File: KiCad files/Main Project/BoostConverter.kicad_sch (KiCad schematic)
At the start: 9 parts, among them Q1 Si2319CDS, U1 2108

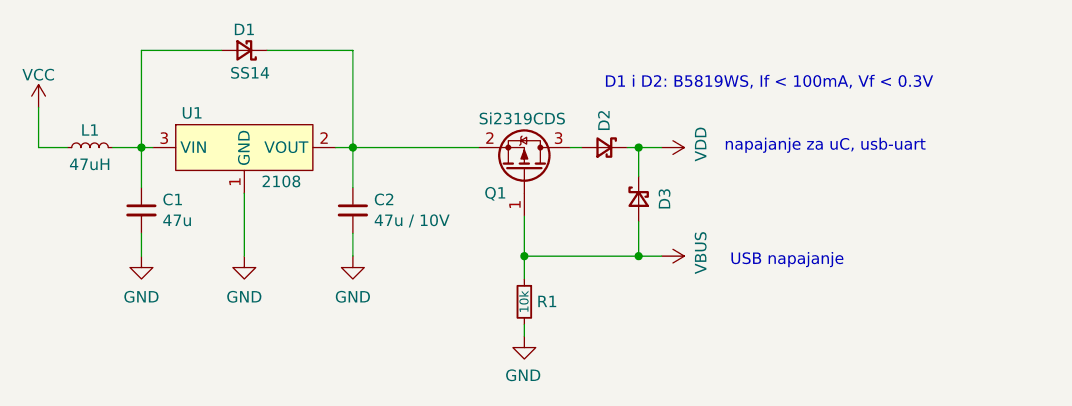
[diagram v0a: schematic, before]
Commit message: update
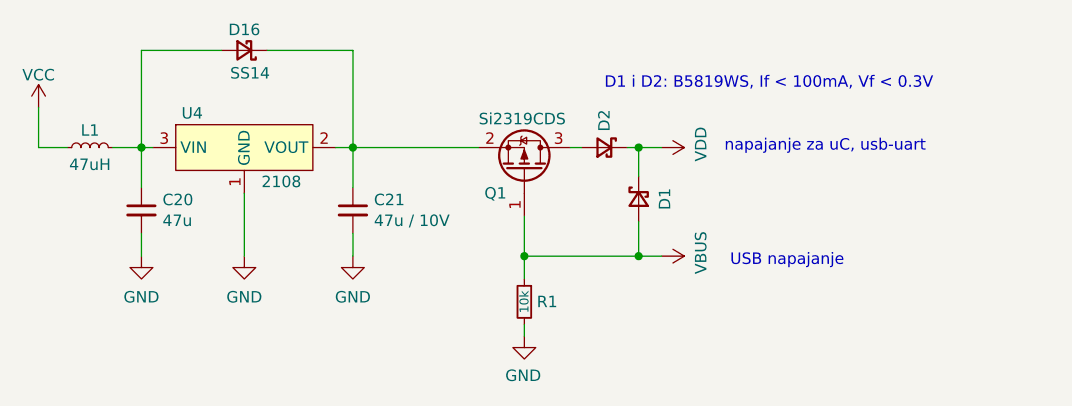
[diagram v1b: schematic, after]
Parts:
- renumbered C1 to C20, C2 to C21, D3 to D1, D1 to D16, U1 to U4
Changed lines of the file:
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@@
   (symbol (lib_id "power:VBUS") (at 139.065 93.345 270) (mirror x) (unit 1)
     (in_bom yes) (on_board yes)
-    (property "Reference" "#PWR09" (id 0) (at 135.255 93.345 0)
+    (property "Reference" "#PWR01" (id 0) (at 135.255 93.345 0)
       (effects (font (size 1.27 1.27)) hide)
     )
@@
   (symbol (lib_id "Device:D_Schottky_Small") (at 136.525 86.995 90) (mirror x) (unit 1)
     (in_bom yes) (on_board yes)
-    (property "Reference" "D3" (id 0) (at 139.446 86.995 0))
+    (property "Reference" "D1" (id 0) (at 139.446 86.995 0))
     (property "Value" "B5819WS" (id 1) (at 139.4714 86.995 0)
       (effects (font (size 1.27 1.27)) hide)
@@
   (symbol (lib_id "power:GND") (at 123.825 102.235 0) (mirror y) (unit 1)
     (in_bom yes) (on_board yes)
-    (property "Reference" "#PWR010" (id 0) (at 123.825 108.585 0)
+    (property "Reference" "#PWR02" (id 0) (at 123.825 108.585 0)
       (effects (font (size 1.27 1.27)) hide)
     )
@@
   (symbol (lib_id "power:VDD") (at 139.065 81.28 270) (mirror x) (unit 1)
     (in_bom yes) (on_board yes)
-    (property "Reference" "#PWR05" (id 0) (at 135.255 81.28 0)
+    (property "Reference" "#PWR03" (id 0) (at 135.255 81.28 0)
       (effects (font (size 1.27 1.27)) hide)
     )
@@
   (symbol (lib_id "power:GND") (at 81.28 93.345 0) (unit 1)
     (in_bom yes) (on_board yes) (fields_autoplaced)
-    (property "Reference" "#PWR06" (id 0) (at 81.28 99.695 0)
+    (property "Reference" "#PWR0101" (id 0) (at 81.28 99.695 0)
       (effects (font (size 1.27 1.27)) hide)
     )
@@
   (symbol (lib_id "power:VCC") (at 69.85 76.835 0) (unit 1)
     (in_bom yes) (on_board yes) (fields_autoplaced)
-    (property "Reference" "#PWR04" (id 0) (at 69.85 80.645 0)
+    (property "Reference" "#PWR0102" (id 0) (at 69.85 80.645 0)
       (effects (font (size 1.27 1.27)) hide)
     )
@@
   (symbol (lib_id "power:GND") (at 104.775 93.345 0) (unit 1)
     (in_bom yes) (on_board yes) (fields_autoplaced)
-    (property "Reference" "#PWR08" (id 0) (at 104.775 99.695 0)
+    (property "Reference" "#PWR0104" (id 0) (at 104.775 99.695 0)
       (effects (font (size 1.27 1.27)) hide)
     )
@@
   (symbol (lib_id "CNLJS-symbols:2108") (at 92.71 81.28 0) (unit 1)
     (in_bom yes) (on_board yes)
-    (property "Reference" "U1" (id 0) (at 85.725 77.47 0)
+    (property "Reference" "U4" (id 0) (at 85.725 77.47 0)
       (effects (font (size 1.27 1.27)) (justify left))
     )
@@
   (symbol (lib_id "power:GND") (at 92.71 93.345 0) (unit 1)
     (in_bom yes) (on_board yes) (fields_autoplaced)
-    (property "Reference" "#PWR07" (id 0) (at 92.71 99.695 0)
+    (property "Reference" "#PWR0103" (id 0) (at 92.71 99.695 0)
       (effects (font (size 1.27 1.27)) hide)
     )
@@
   (symbol (lib_id "Device:C_Small") (at 104.775 88.265 0) (unit 1)
     (in_bom yes) (on_board yes)
-    (property "Reference" "C2" (id 0) (at 107.1118 87.0966 0)
+    (property "Reference" "C21" (id 0) (at 107.1118 87.0966 0)
       (effects (font (size 1.27 1.27)) (justify left))
     )
@@
   (symbol (lib_id "Device:C_Small") (at 81.28 88.265 0) (unit 1)
     (in_bom yes) (on_board yes)
-    (property "Reference" "C1" (id 0) (at 83.6168 87.0966 0)
+    (property "Reference" "C20" (id 0) (at 83.6168 87.0966 0)
       (effects (font (size 1.27 1.27)) (justify left))
     )
@@
   (symbol (lib_id "Device:D_Schottky_Small") (at 92.71 70.485 180) (unit 1)
     (in_bom yes) (on_board yes)
-    (property "Reference" "D1" (id 0) (at 92.71 68.199 0))
+    (property "Reference" "D16" (id 0) (at 92.71 68.199 0))
     (property "Value" "SS14" (id 1) (at 93.345 73.025 0))
     (property "Footprint" "Diode_SMD:D_SMA" (id 2) (at 92.71 70.485 90)

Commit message: shematic update
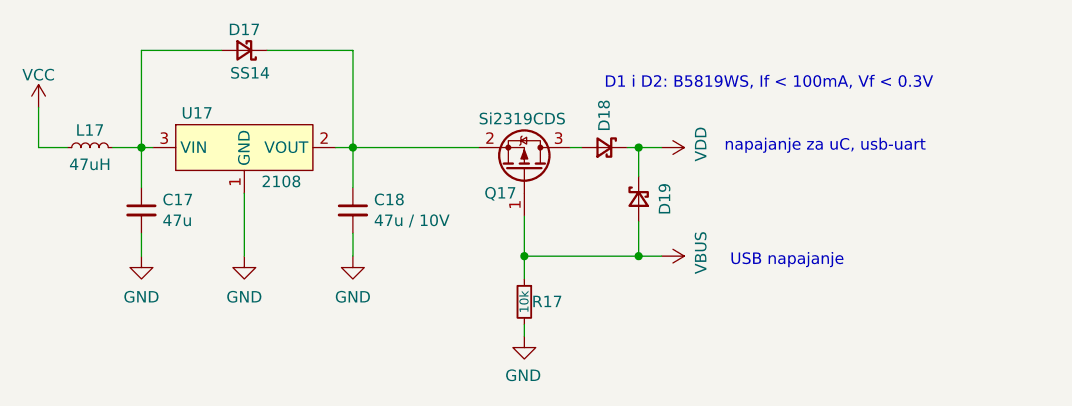
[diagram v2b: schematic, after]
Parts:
- renumbered C20 to C17, C21 to C18, D16 to D17, D2 to D18, D1 to D19, L1 to L17, Q1 to Q17, R1 to R17, U4 to U17
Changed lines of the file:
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@@
   (symbol (lib_id "power:VBUS") (at 139.065 93.345 270) (mirror x) (unit 1)
     (in_bom yes) (on_board yes)
-    (property "Reference" "#PWR01" (id 0) (at 135.255 93.345 0)
+    (property "Reference" "#PWR025" (id 0) (at 135.255 93.345 0)
       (effects (font (size 1.27 1.27)) hide)
     )
@@
   (symbol (lib_id "Device:D_Schottky_Small") (at 136.525 86.995 90) (mirror x) (unit 1)
     (in_bom yes) (on_board yes)
-    (property "Reference" "D1" (id 0) (at 139.446 86.995 0))
+    (property "Reference" "D19" (id 0) (at 139.446 86.995 0))
     (property "Value" "B5819WS" (id 1) (at 139.4714 86.995 0)
       (effects (font (size 1.27 1.27)) hide)
@@
   (symbol (lib_id "Device:R_Small") (at 123.825 98.425 0) (mirror y) (unit 1)
     (in_bom yes) (on_board yes)
-    (property "Reference" "R1" (id 0) (at 126.365 98.425 0))
+    (property "Reference" "R17" (id 0) (at 126.365 98.425 0))
     (property "Value" "10k" (id 1) (at 123.825 98.425 90)
       (effects (font (size 0.9906 0.9906)))
@@
   (symbol (lib_id "power:GND") (at 123.825 102.235 0) (mirror y) (unit 1)
     (in_bom yes) (on_board yes)
-    (property "Reference" "#PWR02" (id 0) (at 123.825 108.585 0)
+    (property "Reference" "#PWR026" (id 0) (at 123.825 108.585 0)
       (effects (font (size 1.27 1.27)) hide)
     )
@@
   (symbol (lib_id "Transistor_FET:Si2319CDS") (at 123.825 83.82 270) (mirror x) (unit 1)
     (in_bom yes) (on_board yes)
-    (property "Reference" "Q1" (id 0) (at 119.38 86.36 90)
+    (property "Reference" "Q17" (id 0) (at 119.38 86.36 90)
       (effects (font (size 1.27 1.27)) (justify left))
     )
@@
   (symbol (lib_id "Device:D_Schottky_Small") (at 132.715 81.28 0) (mirror y) (unit 1)
     (in_bom yes) (on_board yes)
-    (property "Reference" "D2" (id 0) (at 132.715 79.502 90)
+    (property "Reference" "D18" (id 0) (at 132.715 79.502 90)
       (effects (font (size 1.27 1.27)) (justify left))
     )
@@
   (symbol (lib_id "power:VDD") (at 139.065 81.28 270) (mirror x) (unit 1)
     (in_bom yes) (on_board yes)
-    (property "Reference" "#PWR03" (id 0) (at 135.255 81.28 0)
+    (property "Reference" "#PWR021" (id 0) (at 135.255 81.28 0)
       (effects (font (size 1.27 1.27)) hide)
     )
@@
   (symbol (lib_id "power:GND") (at 81.28 93.345 0) (unit 1)
     (in_bom yes) (on_board yes) (fields_autoplaced)
-    (property "Reference" "#PWR0101" (id 0) (at 81.28 99.695 0)
+    (property "Reference" "#PWR022" (id 0) (at 81.28 99.695 0)
       (effects (font (size 1.27 1.27)) hide)
     )
@@
   (symbol (lib_id "Device:L_Small") (at 75.565 81.28 90) (unit 1)
     (in_bom yes) (on_board yes)
-    (property "Reference" "L1" (id 0) (at 75.565 79.375 90))
+    (property "Reference" "L17" (id 0) (at 75.565 79.375 90))
     (property "Value" "47uH" (id 1) (at 75.565 83.185 90))
     (property "Footprint" "CNLJS:L_Taiyo-Yuden_NR-50xx" (id 2) (at 75.565 81.28 0)
@@
   (symbol (lib_id "power:VCC") (at 69.85 76.835 0) (unit 1)
     (in_bom yes) (on_board yes) (fields_autoplaced)
-    (property "Reference" "#PWR0102" (id 0) (at 69.85 80.645 0)
+    (property "Reference" "#PWR020" (id 0) (at 69.85 80.645 0)
       (effects (font (size 1.27 1.27)) hide)
     )
@@
   (symbol (lib_id "power:GND") (at 104.775 93.345 0) (unit 1)
     (in_bom yes) (on_board yes) (fields_autoplaced)
-    (property "Reference" "#PWR0104" (id 0) (at 104.775 99.695 0)
+    (property "Reference" "#PWR024" (id 0) (at 104.775 99.695 0)
       (effects (font (size 1.27 1.27)) hide)
     )
@@
   (symbol (lib_id "CNLJS-symbols:2108") (at 92.71 81.28 0) (unit 1)
     (in_bom yes) (on_board yes)
-    (property "Reference" "U4" (id 0) (at 85.725 77.47 0)
+    (property "Reference" "U17" (id 0) (at 85.725 77.47 0)
       (effects (font (size 1.27 1.27)) (justify left))
     )
@@
   (symbol (lib_id "power:GND") (at 92.71 93.345 0) (unit 1)
     (in_bom yes) (on_board yes) (fields_autoplaced)
-    (property "Reference" "#PWR0103" (id 0) (at 92.71 99.695 0)
+    (property "Reference" "#PWR023" (id 0) (at 92.71 99.695 0)
       (effects (font (size 1.27 1.27)) hide)
     )
@@
   (symbol (lib_id "Device:C_Small") (at 104.775 88.265 0) (unit 1)
     (in_bom yes) (on_board yes)
-    (property "Reference" "C21" (id 0) (at 107.1118 87.0966 0)
+    (property "Reference" "C18" (id 0) (at 107.1118 87.0966 0)
       (effects (font (size 1.27 1.27)) (justify left))
     )
@@
   (symbol (lib_id "Device:C_Small") (at 81.28 88.265 0) (unit 1)
     (in_bom yes) (on_board yes)
-    (property "Reference" "C20" (id 0) (at 83.6168 87.0966 0)
+    (property "Reference" "C17" (id 0) (at 83.6168 87.0966 0)
       (effects (font (size 1.27 1.27)) (justify left))
     )
@@
   (symbol (lib_id "Device:D_Schottky_Small") (at 92.71 70.485 180) (unit 1)
     (in_bom yes) (on_board yes)
-    (property "Reference" "D16" (id 0) (at 92.71 68.199 0))
+    (property "Reference" "D17" (id 0) (at 92.71 68.199 0))
     (property "Value" "SS14" (id 1) (at 93.345 73.025 0))
     (property "Footprint" "Diode_SMD:D_SMA" (id 2) (at 92.71 70.485 90)

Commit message: update
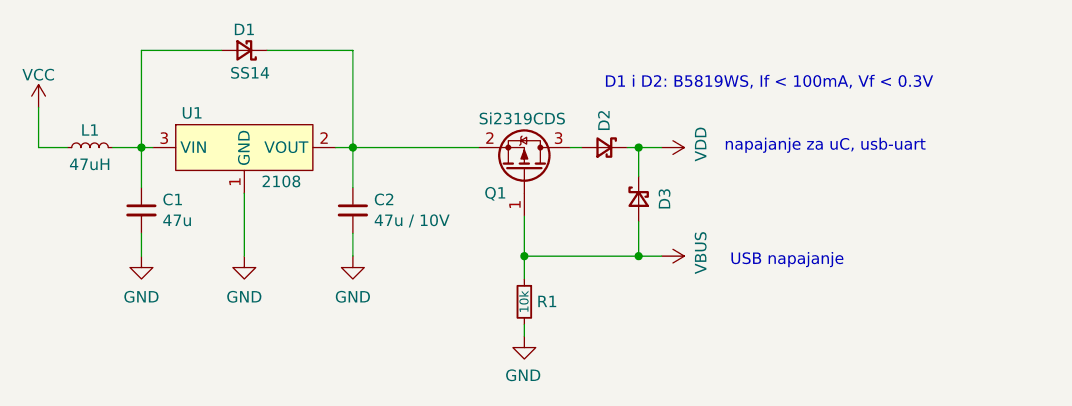
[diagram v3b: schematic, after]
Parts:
- renumbered C17 to C1, C18 to C2, D17 to D1, D18 to D2, D19 to D3, L17 to L1, Q17 to Q1, R17 to R1, U17 to U1
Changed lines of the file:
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@@
   (symbol (lib_id "power:VBUS") (at 139.065 93.345 270) (mirror x) (unit 1)
     (in_bom yes) (on_board yes)
-    (property "Reference" "#PWR025" (id 0) (at 135.255 93.345 0)
+    (property "Reference" "#PWR09" (id 0) (at 135.255 93.345 0)
       (effects (font (size 1.27 1.27)) hide)
     )
@@
   (symbol (lib_id "Device:D_Schottky_Small") (at 136.525 86.995 90) (mirror x) (unit 1)
     (in_bom yes) (on_board yes)
-    (property "Reference" "D19" (id 0) (at 139.446 86.995 0))
+    (property "Reference" "D3" (id 0) (at 139.446 86.995 0))
     (property "Value" "B5819WS" (id 1) (at 139.4714 86.995 0)
       (effects (font (size 1.27 1.27)) hide)
@@
   (symbol (lib_id "Device:R_Small") (at 123.825 98.425 0) (mirror y) (unit 1)
     (in_bom yes) (on_board yes)
-    (property "Reference" "R17" (id 0) (at 126.365 98.425 0))
+    (property "Reference" "R1" (id 0) (at 126.365 98.425 0))
     (property "Value" "10k" (id 1) (at 123.825 98.425 90)
       (effects (font (size 0.9906 0.9906)))
@@
   (symbol (lib_id "power:GND") (at 123.825 102.235 0) (mirror y) (unit 1)
     (in_bom yes) (on_board yes)
-    (property "Reference" "#PWR026" (id 0) (at 123.825 108.585 0)
+    (property "Reference" "#PWR010" (id 0) (at 123.825 108.585 0)
       (effects (font (size 1.27 1.27)) hide)
     )
@@
   (symbol (lib_id "Transistor_FET:Si2319CDS") (at 123.825 83.82 270) (mirror x) (unit 1)
     (in_bom yes) (on_board yes)
-    (property "Reference" "Q17" (id 0) (at 119.38 86.36 90)
+    (property "Reference" "Q1" (id 0) (at 119.38 86.36 90)
       (effects (font (size 1.27 1.27)) (justify left))
     )
@@
   (symbol (lib_id "Device:D_Schottky_Small") (at 132.715 81.28 0) (mirror y) (unit 1)
     (in_bom yes) (on_board yes)
-    (property "Reference" "D18" (id 0) (at 132.715 79.502 90)
+    (property "Reference" "D2" (id 0) (at 132.715 79.502 90)
       (effects (font (size 1.27 1.27)) (justify left))
     )
@@
   (symbol (lib_id "power:VDD") (at 139.065 81.28 270) (mirror x) (unit 1)
     (in_bom yes) (on_board yes)
-    (property "Reference" "#PWR021" (id 0) (at 135.255 81.28 0)
+    (property "Reference" "#PWR05" (id 0) (at 135.255 81.28 0)
       (effects (font (size 1.27 1.27)) hide)
     )
@@
   (symbol (lib_id "power:GND") (at 81.28 93.345 0) (unit 1)
     (in_bom yes) (on_board yes) (fields_autoplaced)
-    (property "Reference" "#PWR022" (id 0) (at 81.28 99.695 0)
+    (property "Reference" "#PWR06" (id 0) (at 81.28 99.695 0)
       (effects (font (size 1.27 1.27)) hide)
     )
@@
   (symbol (lib_id "Device:L_Small") (at 75.565 81.28 90) (unit 1)
     (in_bom yes) (on_board yes)
-    (property "Reference" "L17" (id 0) (at 75.565 79.375 90))
+    (property "Reference" "L1" (id 0) (at 75.565 79.375 90))
     (property "Value" "47uH" (id 1) (at 75.565 83.185 90))
     (property "Footprint" "CNLJS:L_Taiyo-Yuden_NR-50xx" (id 2) (at 75.565 81.28 0)
@@
   (symbol (lib_id "power:VCC") (at 69.85 76.835 0) (unit 1)
     (in_bom yes) (on_board yes) (fields_autoplaced)
-    (property "Reference" "#PWR020" (id 0) (at 69.85 80.645 0)
+    (property "Reference" "#PWR04" (id 0) (at 69.85 80.645 0)
       (effects (font (size 1.27 1.27)) hide)
     )
@@
   (symbol (lib_id "power:GND") (at 104.775 93.345 0) (unit 1)
     (in_bom yes) (on_board yes) (fields_autoplaced)
-    (property "Reference" "#PWR024" (id 0) (at 104.775 99.695 0)
+    (property "Reference" "#PWR08" (id 0) (at 104.775 99.695 0)
       (effects (font (size 1.27 1.27)) hide)
     )
@@
   (symbol (lib_id "CNLJS-symbols:2108") (at 92.71 81.28 0) (unit 1)
     (in_bom yes) (on_board yes)
-    (property "Reference" "U17" (id 0) (at 85.725 77.47 0)
+    (property "Reference" "U1" (id 0) (at 85.725 77.47 0)
       (effects (font (size 1.27 1.27)) (justify left))
     )
@@
   (symbol (lib_id "power:GND") (at 92.71 93.345 0) (unit 1)
     (in_bom yes) (on_board yes) (fields_autoplaced)
-    (property "Reference" "#PWR023" (id 0) (at 92.71 99.695 0)
+    (property "Reference" "#PWR07" (id 0) (at 92.71 99.695 0)
       (effects (font (size 1.27 1.27)) hide)
     )
@@
   (symbol (lib_id "Device:C_Small") (at 104.775 88.265 0) (unit 1)
     (in_bom yes) (on_board yes)
-    (property "Reference" "C18" (id 0) (at 107.1118 87.0966 0)
+    (property "Reference" "C2" (id 0) (at 107.1118 87.0966 0)
       (effects (font (size 1.27 1.27)) (justify left))
     )
@@
   (symbol (lib_id "Device:C_Small") (at 81.28 88.265 0) (unit 1)
     (in_bom yes) (on_board yes)
-    (property "Reference" "C17" (id 0) (at 83.6168 87.0966 0)
+    (property "Reference" "C1" (id 0) (at 83.6168 87.0966 0)
       (effects (font (size 1.27 1.27)) (justify left))
     )
@@
   (symbol (lib_id "Device:D_Schottky_Small") (at 92.71 70.485 180) (unit 1)
     (in_bom yes) (on_board yes)
-    (property "Reference" "D17" (id 0) (at 92.71 68.199 0))
+    (property "Reference" "D1" (id 0) (at 92.71 68.199 0))
     (property "Value" "SS14" (id 1) (at 93.345 73.025 0))
     (property "Footprint" "Diode_SMD:D_SMA" (id 2) (at 92.71 70.485 90)
